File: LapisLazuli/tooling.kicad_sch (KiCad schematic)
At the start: 71 parts, among them J1 Conn_01x02, J10 Conn_01x03, J11 Conn_01x03, J12 Conn_01x02, J13 Conn_01x02, J14 Conn_01x04, J15 Conn_01x04, J16 Conn_01x02, J2 Conn_01x02, J3 Conn_01x02, J4 Conn_01x02, J5 Conn_01x02, J6 Conn_01x02, J7 Conn_01x05, J8 Conn_01x03, J9 Conn_01x03, U1 DRV8231ADSG, U13 LTC4311CSC6-TRPBF, U14 TCA9546APWR, U2 NC7SZ18P6X, U3 DRV8231ADSG, U4 NC7SZ18P6X, U5 DRV8231ADSG, U6 DRV8231ADSG, U7 NC7SZ18P6X, U8 NC7SZ18P6X, U9 ISO1412DW

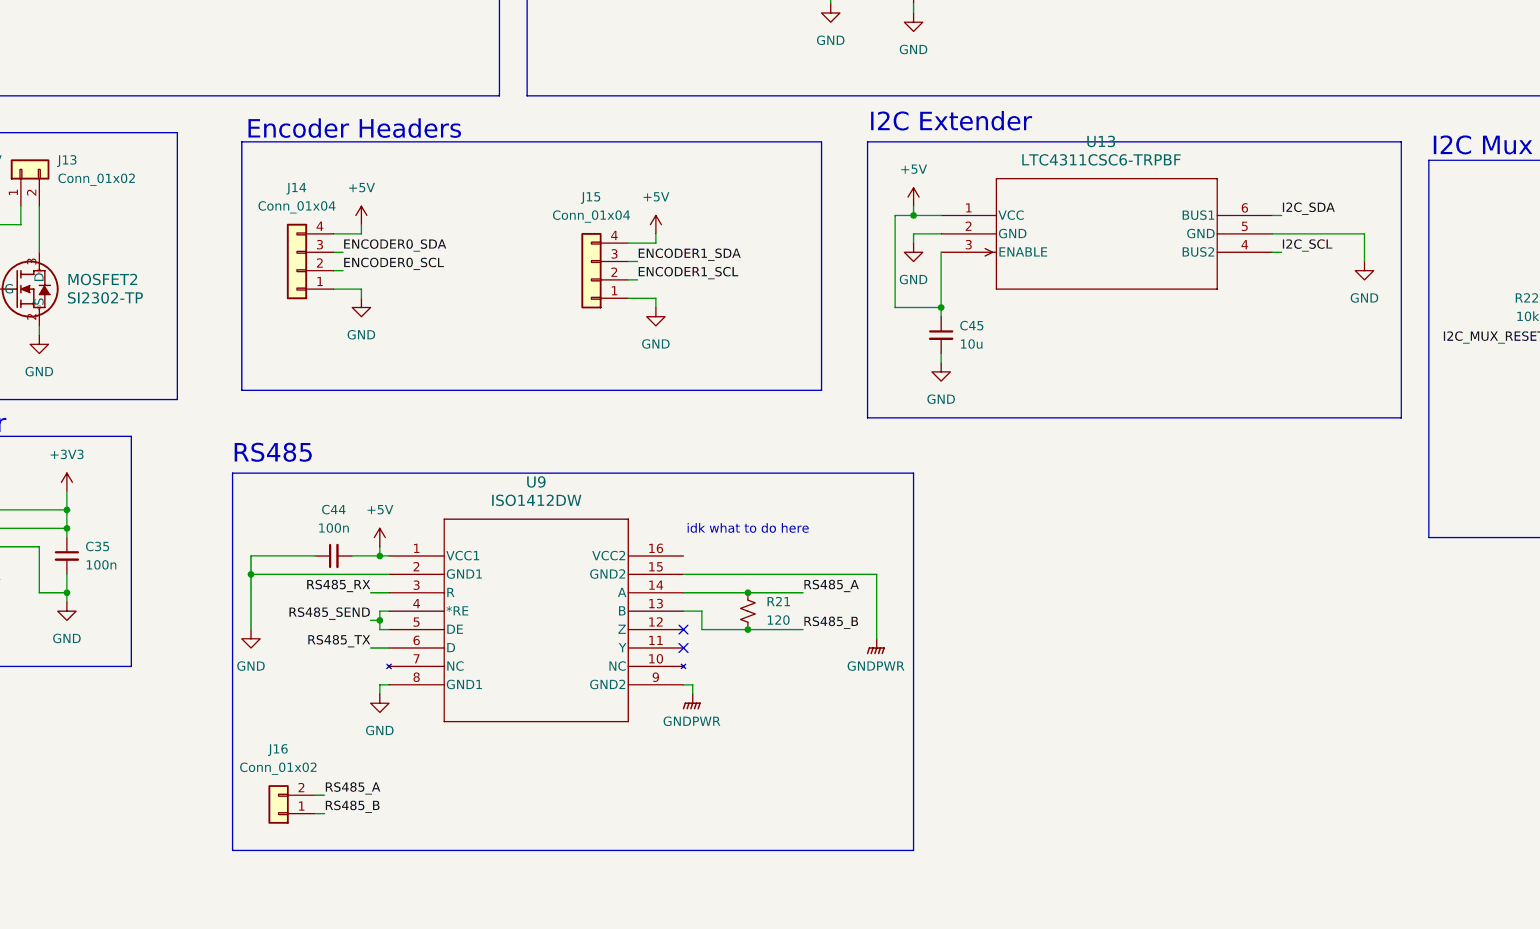
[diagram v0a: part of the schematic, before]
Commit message: Most footprints and second I2C extender
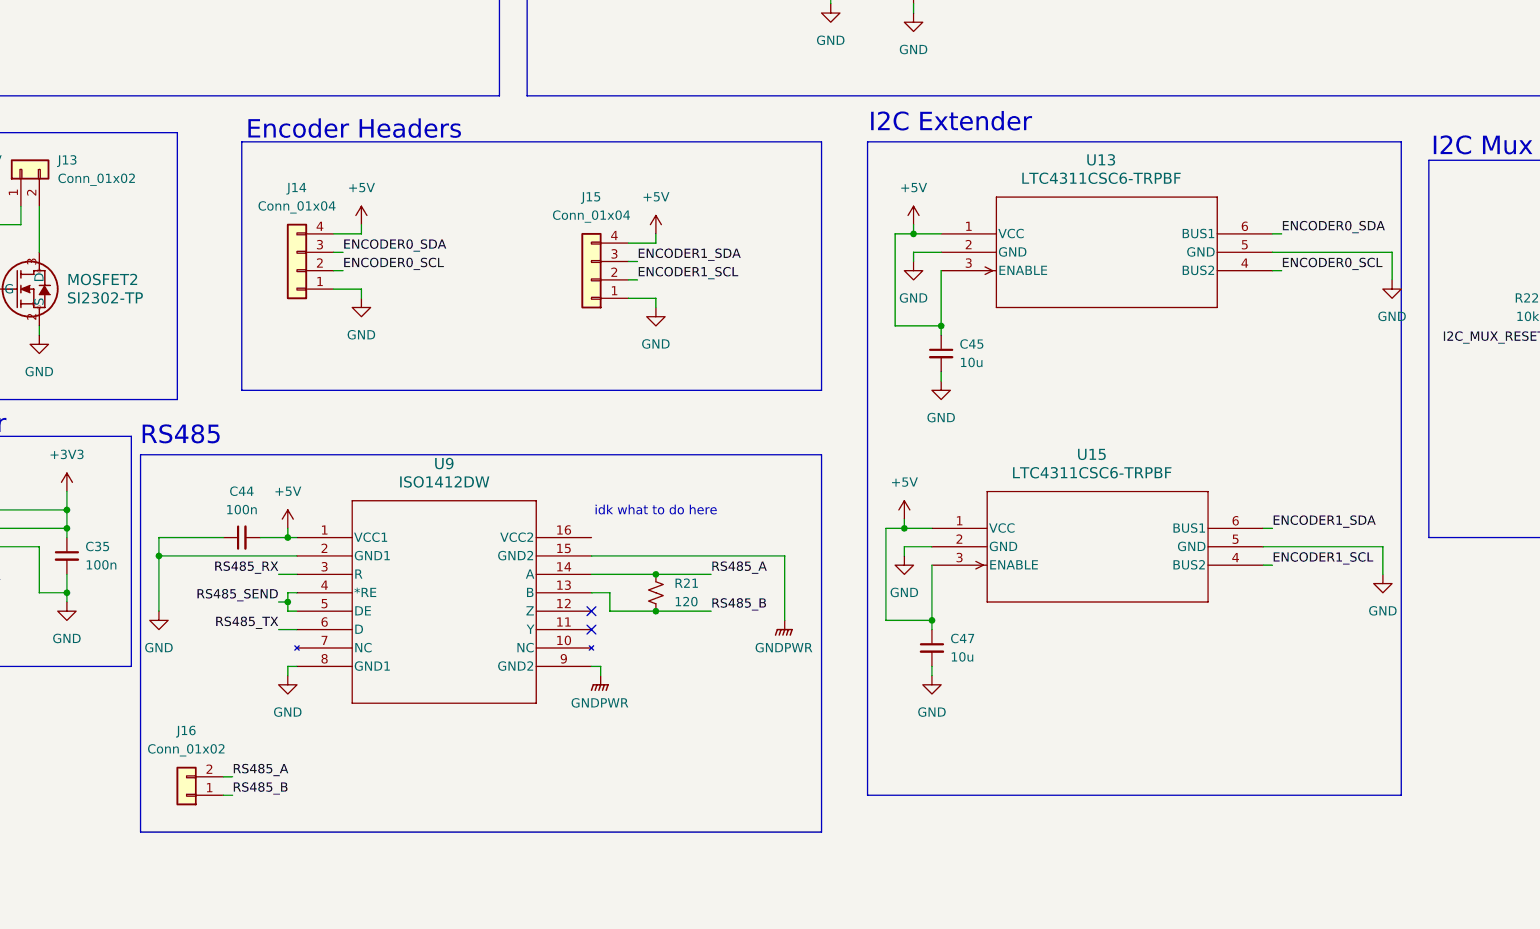
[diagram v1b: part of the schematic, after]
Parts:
- added C47: 10u, Capacitor_SMD:C_0805_2012Metric, symbol Device:C_Small
- added U15: LTC4311CSC6-TRPBF, Package_TO_SOT_SMD:SOT-363_SC-70-6, symbol 2025-11-21_17-52-57:LTC4311CSC6-TRPBF
- C1, C10, C13, C14, C15, C16, C2, C35, C37, C39, C4, C41, C43, C44, C46, C5, C7, C8, C9: footprint (none) -> Capacitor_SMD:C_0603_1608Metric; Digikey (none) -> C14663; LCSC (none) -> C14663
- C11, C12, C3, C6: footprint (none) -> Capacitor_SMD:C_0805_2012Metric; Digikey (none) -> C16780; LCSC (none) -> C16780
- C36, C38, C40, C42: footprint (none) -> Capacitor_SMD:CP_Elec_6.3x7.7; Digikey (none) -> C3338; LCSC (none) -> C3338
- C45: footprint (none) -> Capacitor_SMD:C_0805_2012Metric; Digikey (none) -> C19702; LCSC (none) -> C19702
- J1, J12, J13, J16, J2, J3, J4, J5, J6: footprint (none) -> Connector_PinHeader_2.54mm:PinHeader_1x02_P2.54mm_Vertical
- J10, J11, J8, J9: footprint (none) -> Connector_PinHeader_2.54mm:PinHeader_1x03_P2.54mm_Vertical
- J14, J15: footprint (none) -> Connector_PinHeader_2.54mm:PinHeader_1x04_P2.54mm_Vertical
- J7: footprint (none) -> Connector_PinHeader_2.54mm:PinHeader_1x05_P2.54mm_Vertical
- MOSFET1, MOSFET2: footprint SOT-23_MCC -> Package_TO_SOT_SMD:SOT-23; LCSC (none) -> C10488
- R1, R10, R11, R12, R2, R22, R3, R4, R5, R6, R7, R8, R9: footprint (none) -> Resistor_SMD:R_0603_1608Metric; LCSC (none) -> C25804
- R21: footprint (none) -> Resistor_SMD:R_0603_1608Metric; LCSC (none) -> C22787
- U1, U3, U5, U6: LCSC (none) -> C5139865
- U13: footprint SOT-6_SC_LIT -> Package_TO_SOT_SMD:SOT-363_SC-70-6; LCSC (none) -> C580856
- U14: footprint TCA9546APWR:SOP65P640X120-16N -> Package_SO:TSSOP-16_4.4x5mm_P0.65mm; LCSC (none) -> C201653
- U2, U4, U7, U8: footprint SC70-6_2P2X1P35_ONS -> Package_TO_SOT_SMD:SOT-363_SC-70-6; LCSC (none) -> C462890
- U9: footprint DW16_TEX -> Package_SO:SOIC-16W_7.5x10.3mm_P1.27mm; LCSC (none) -> C2672327
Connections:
- net +5V: now also C47.1, U15.1 (VCC), U15.3 (ENABLE)
- net ENCODER0_SCL: now also U13.4 (BUS2)
- net ENCODER0_SDA: now also U13.6 (BUS1)
- net ENCODER1_SCL: now also U15.4 (BUS2)
- net ENCODER1_SDA: now also U15.6 (BUS1)
- net GND: now also C47.2, U15.2 (GND), U15.5 (GND)
- net I2C_SCL: no longer U13.4 (BUS2)
- net I2C_SDA: no longer U13.6 (BUS1)
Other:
- moved on the sheet: C44, C45, J16, R21, U13, U9
